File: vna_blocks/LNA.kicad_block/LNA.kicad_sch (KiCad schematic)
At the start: 12 parts, among them IC5 LVA-273PN+

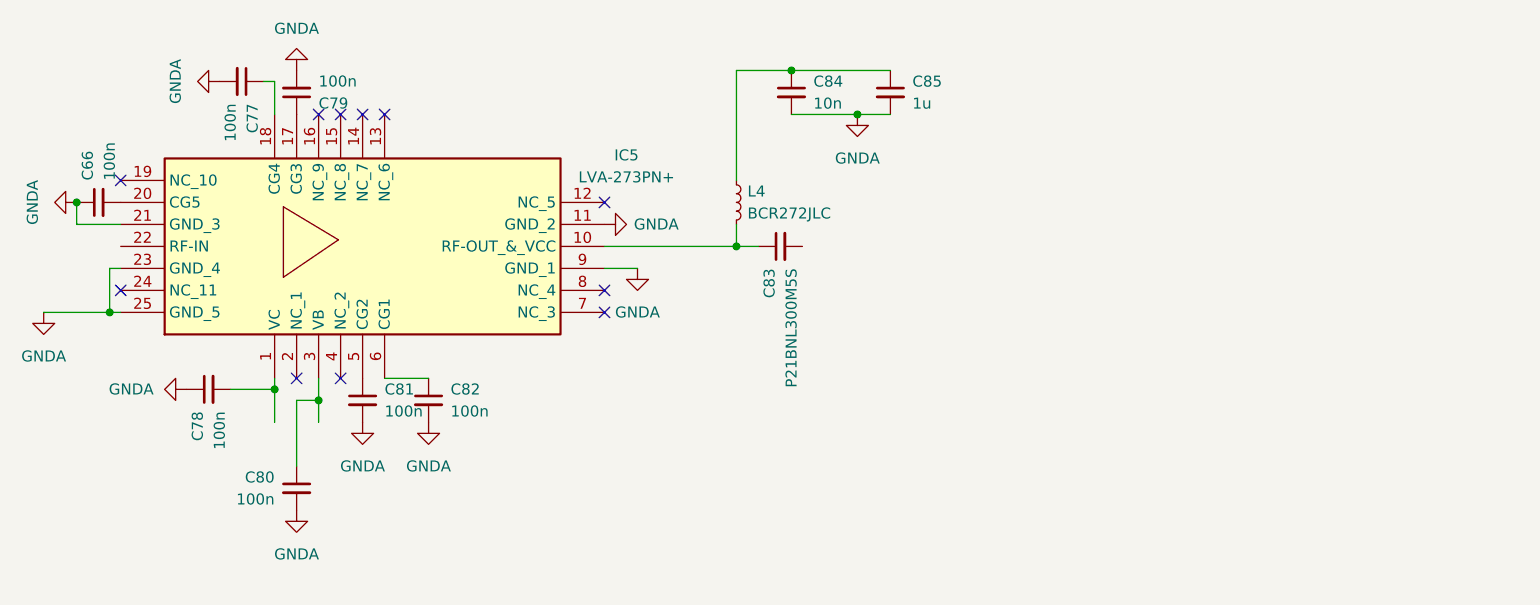
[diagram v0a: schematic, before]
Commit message: new design blocks, footprints
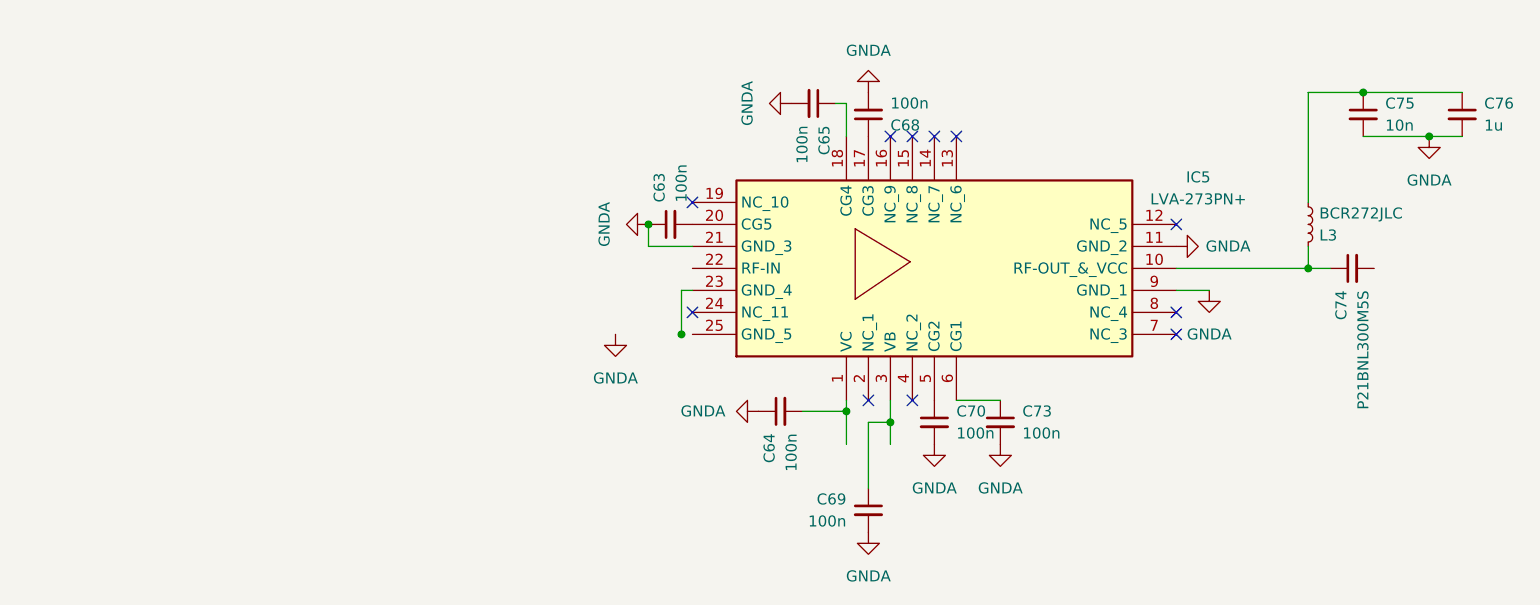
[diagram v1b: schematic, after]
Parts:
- removed C66, C77, C78, C79, C80, C81, C82: 100n, Capacitor_SMD:C_0402_1005Metric, symbol Device:C_Small
- removed C83: P21BNL300M5S, Capacitor_SMD:C_0201_0603Metric, symbol Device:C_Small
- removed C84: 10n, Capacitor_SMD:C_0402_1005Metric, symbol Device:C_Small
- removed C85: 1u, Capacitor_SMD:C_0402_1005Metric, symbol Device:C_Small
- removed L4: BCR272JLC, symbol Device:L_Small
- added C63, C64, C65, C68, C69, C70, C73: 100n, Capacitor_SMD:C_0402_1005Metric, symbol Device:C_Small
- added C74: P21BNL300M5S, Capacitor_SMD:C_0201_0603Metric, symbol Device:C_Small
- added C75: 10n, Capacitor_SMD:C_0402_1005Metric, symbol Device:C_Small
- added C76: 1u, Capacitor_SMD:C_0402_1005Metric, symbol Device:C_Small
- added L3: BCR272JLC, VNA_fp:BCR-272, symbol Device:L_Small
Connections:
- net GNDA: now also C63.1, C64.1, C65.2, C68.2, C69.2, C70.2, C73.2, C75.2, C76.2; no longer IC5.23 (GND_4), IC5.25 (GND_5)
- net at IC5.6 (CG1): now also C73.1
- net at IC5.18 (CG4): now also C65.1
- net at IC5.5 (CG2): now also C70.1
- net at IC5.3 (VB): now also C69.1
- net at IC5.1 (VC): now also C64.2
- net at IC5.17 (CG3): now also C68.1
- net at IC5.10 (RF-OUT_&_VCC): now also C74.1, L3.1
- net at IC5.20 (CG5): now also C63.2
- new net: C75.1, C76.1, L3.2
